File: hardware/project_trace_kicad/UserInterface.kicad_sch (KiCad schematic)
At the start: 13 parts, among them J601 Conn_01x14_Socket, J602 Conn_01x14_Pin, SW601 SW_Push, SW602 SW_Push, SW603 RotaryEncoder, SW604 RotaryEncoder, U601 SBC-OLED01.3

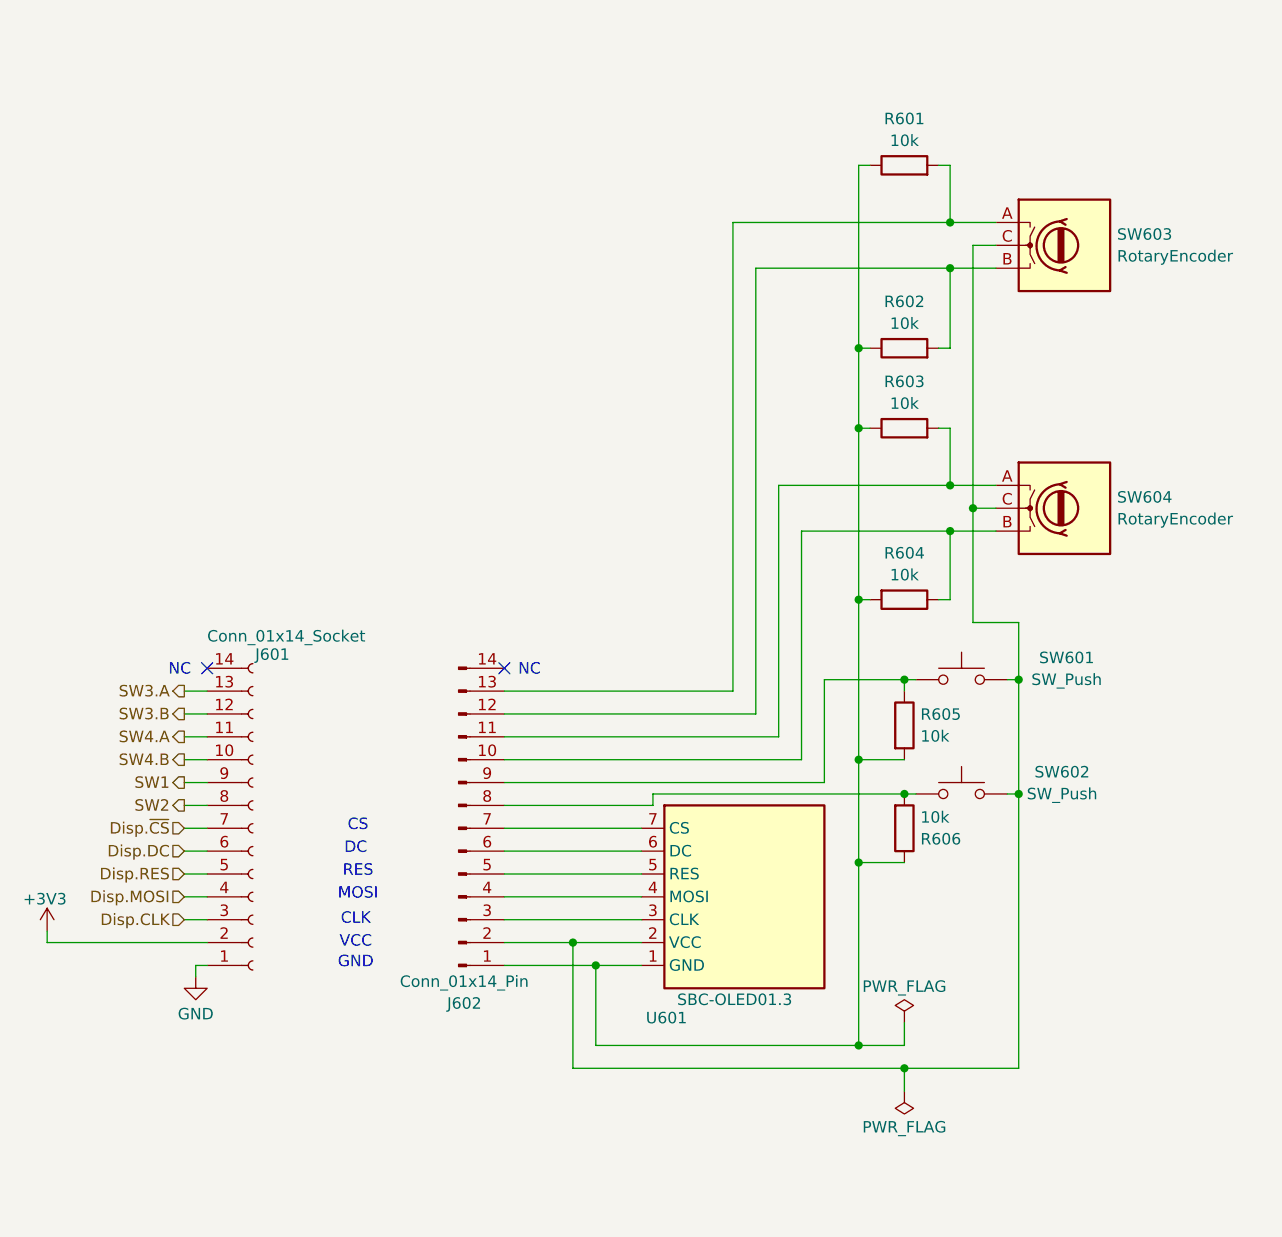
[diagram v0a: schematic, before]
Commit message: Changes to Digital
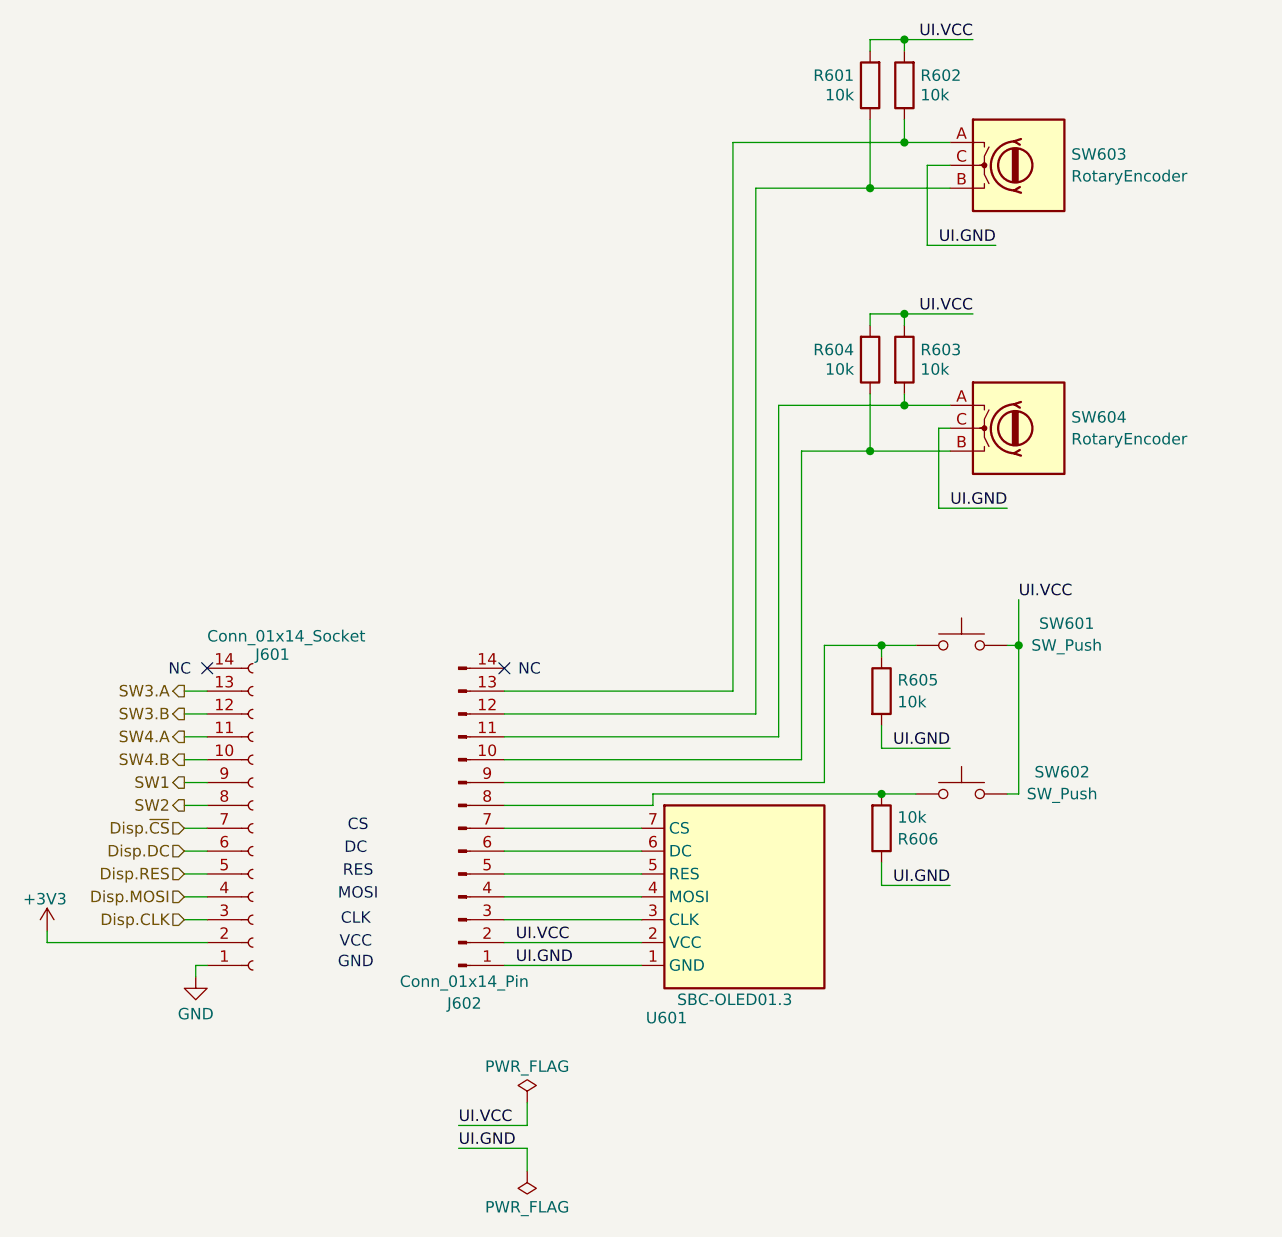
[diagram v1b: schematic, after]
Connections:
- net UI.GND: now reaches J602.1 (Pin_1), R605.2, R606.1, U601.1 (GND)
- net UI.GND: now also SW603.C, SW604.C; no longer R601.1, R602.1, R603.1, R604.2
- net UI.VCC: now reaches J602.2 (Pin_2), SW601.2, SW602.1, U601.2 (VCC)
- net UI.VCC: now also R601.2, R602.2, R603.1, R604.2; no longer SW603.C, SW604.C
- net at J602.12 (Pin_12), SW603.B: now also R601.1; no longer R602.2
- net at J602.13 (Pin_13), SW603.A: now also R602.1; no longer R601.2
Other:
- moved on the sheet: R601, R602, R603, R604, R605, R606, SW601, SW603, SW604
